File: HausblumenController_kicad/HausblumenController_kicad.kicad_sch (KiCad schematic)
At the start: 41 parts, among them J1 Power 12V, J2 Light, J3 Water, J4 Steam, Q1 IRF520N, Q2 IRF520N, Q3 IRF520N, Q4 IRLML0030, SW1 RotaryEncoder_Switch_MP, U1 BlackPill_40pin_SWD, U2 BME280, U3 LM2596S-ADJ, U4 AMS1117

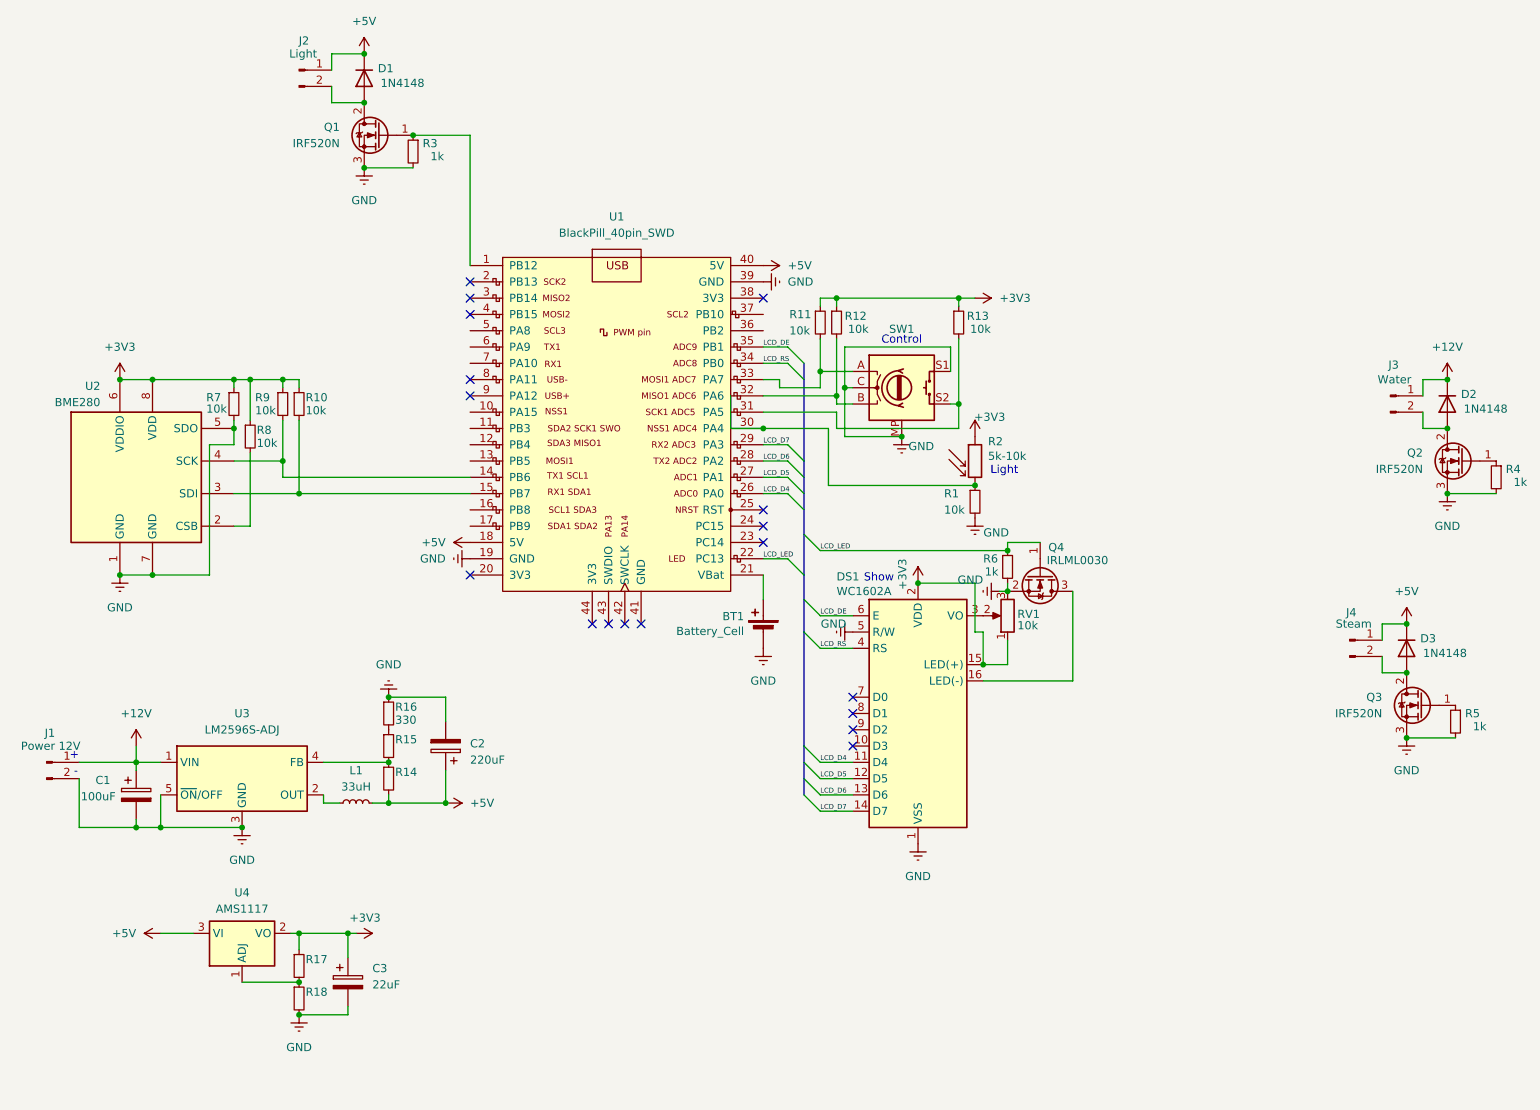
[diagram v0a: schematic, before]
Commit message: chore: naming GPIO
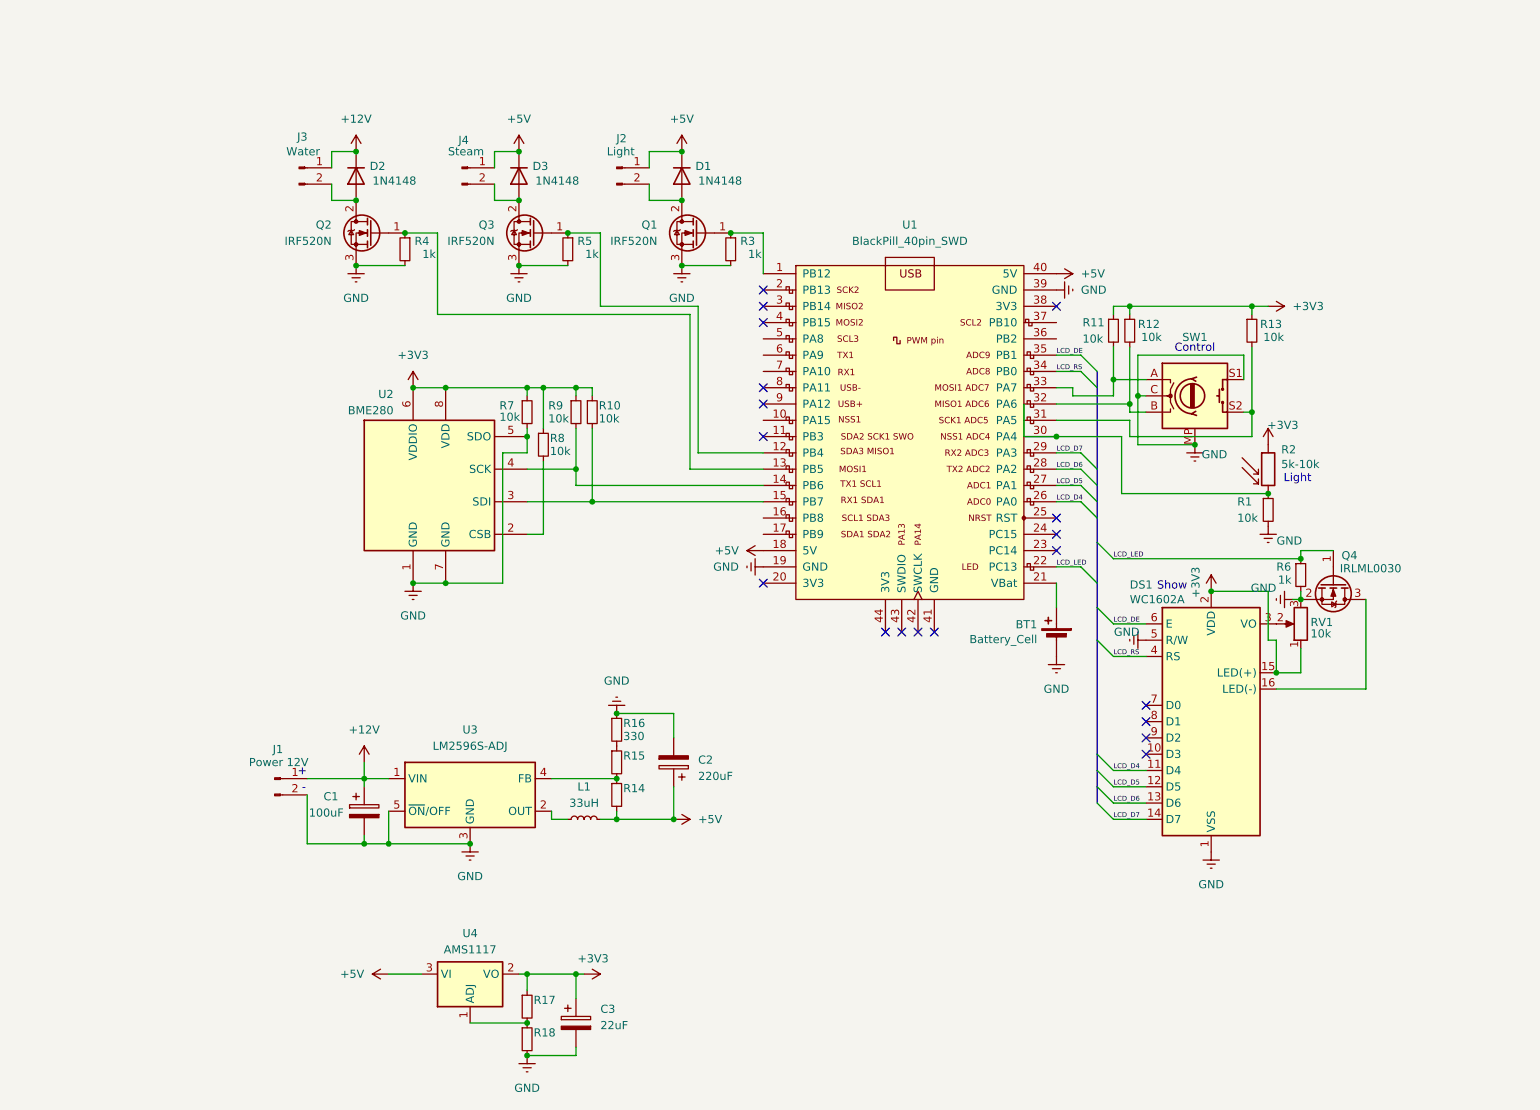
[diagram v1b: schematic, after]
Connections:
- net at Q2.1 (G), R4.1: now also U1.13 (PB5)
- net at U1.12 (PB4): now also Q3.1 (G), R5.1
- no-connect marks 18 -> 19
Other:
- moved on the sheet: BT1, C1, C2, C3, D1, D2, D3, DS1, J1, J2, J3, J4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
